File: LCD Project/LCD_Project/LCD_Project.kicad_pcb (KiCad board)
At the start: 2 copper layers, 109 x 88.5 mm, 6 parts, among them J1 DT15-4P, U1 Teensy4.0, U2 MIC5365-1.3YC5-TR

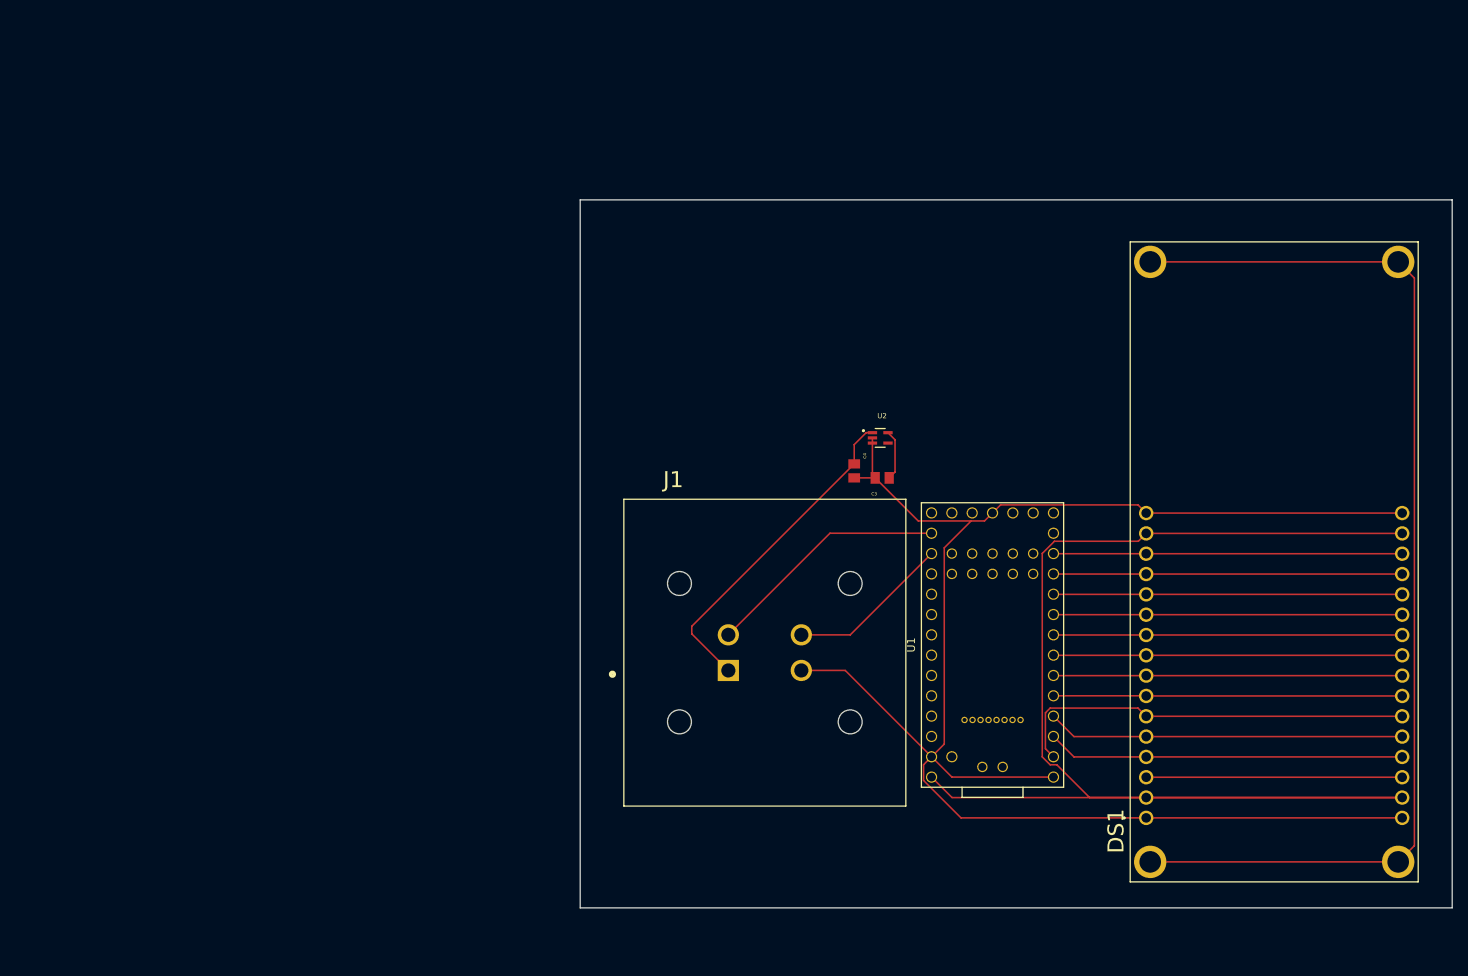
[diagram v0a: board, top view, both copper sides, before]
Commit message: Add files via upload
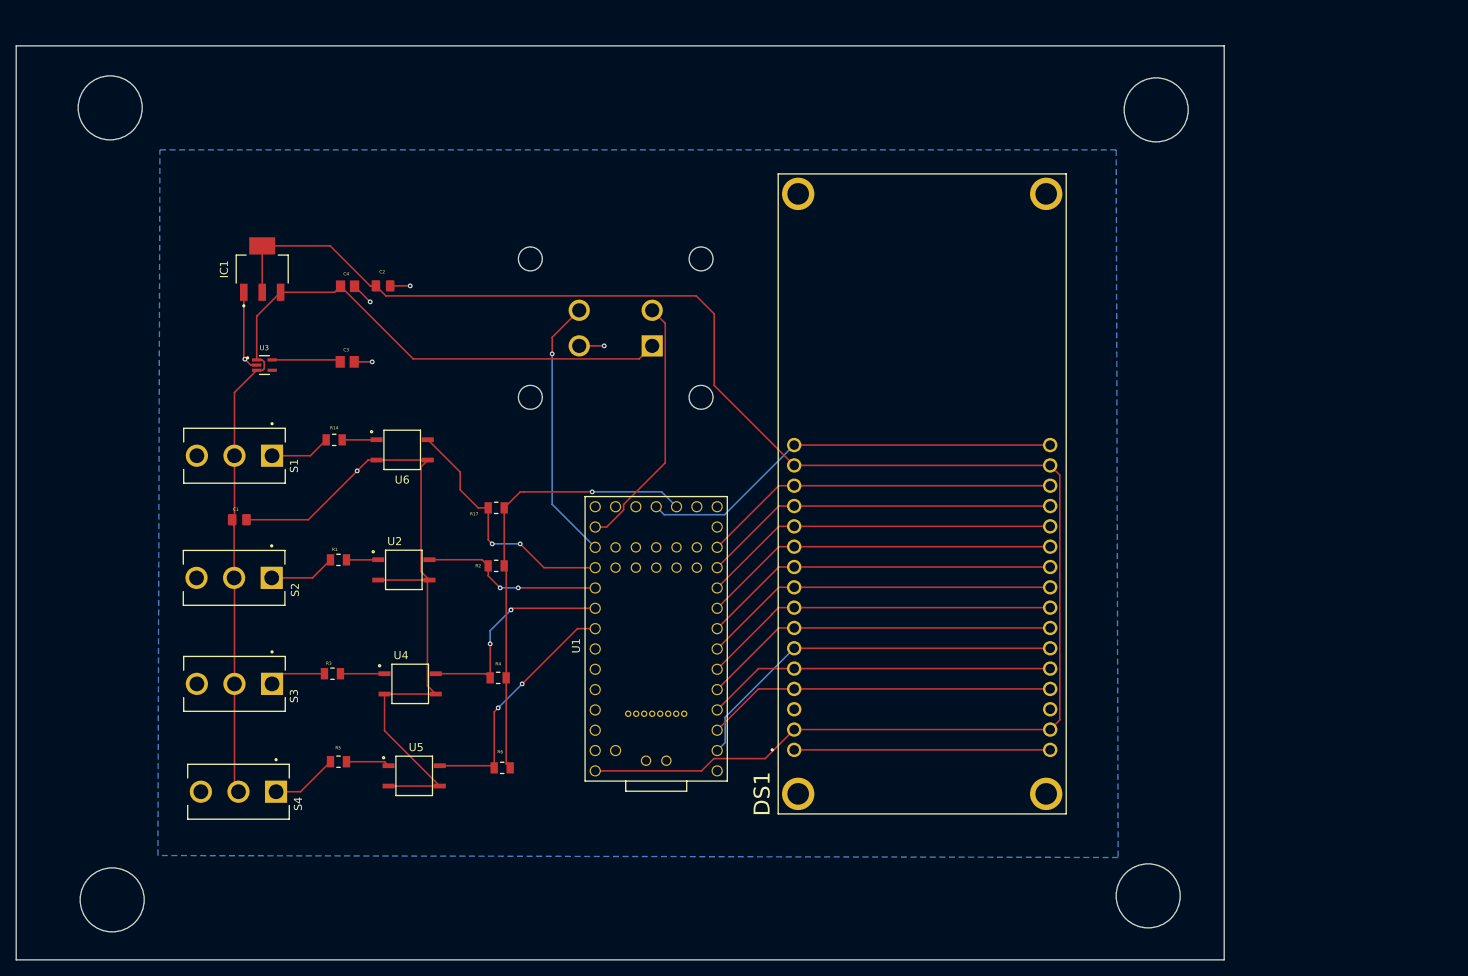
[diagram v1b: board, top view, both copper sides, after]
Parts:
- added C1: CL21A106KOQNNNE, CL21A106KOQNNNE:CAPC2012X140N, F.Cu at (102.4, 84.5)
- added C2: CL21A106KOQNNNE, CL21A106KOQNNNE:CAPC2012X140N, F.Cu at (120.4, 55.2)
- added IC1: REG1117-5, REG1117-5:SOT230P700X180-4N, F.Cu at (105.2, 53.1)
- added R1: 10K, CRCW08051K00FKEA:RESC2012X50N, F.Cu at (114.8, 89.5)
- added R14: 10K, CRCW08051K00FKEA:RESC2012X50N, F.Cu at (114.2, 74.5)
- added R17: 10K, CRCW08051K00FKEA:RESC2012X50N, F.Cu at (134.5, 83.0)
- added R2: 10K, CRCW08051K00FKEA:RESC2012X50N, F.Cu at (134.5, 90.2)
- added R3: 10K, CRCW08051K00FKEA:RESC2012X50N, F.Cu at (114.0, 103.7)
- added R4: 10K, CRCW08051K00FKEA:RESC2012X50N, F.Cu at (134.8, 104.2)
- added R5: 10K, CRCW08051K00FKEA:RESC2012X50N, F.Cu at (114.8, 114.7)
- added R6: 10K, CRCW08051K00FKEA:RESC2012X50N, F.Cu at (135.2, 115.5)
- added S1: 100SP1T1B4M2QE, 100SP1T1B4M2QE:SW_100SP1T1B4M2QE, F.Cu at (101.8, 76.5)
- added S2: 100SP1T1B4M2QE, 100SP1T1B4M2QE:SW_100SP1T1B4M2QE, F.Cu at (101.7, 91.8)
- added S3: 100SP1T1B4M2QE, 100SP1T1B4M2QE:SW_100SP1T1B4M2QE, F.Cu at (101.8, 105.0)
- added S4: 100SP1T1B4M2QE, 100SP1T1B4M2QE:SW_100SP1T1B4M2QE, F.Cu at (102.3, 118.5)
- added U3: MIC5365-1.3YC5-TR, MIC5365-1.3YC5-TR:SOT65P210X110-5N, F.Cu at (105.5, 65.2)
- added U4: VOM618A-3T, VOM618A-3T:SOIC254P695X242-4N, F.Cu at (123.8, 105.0)
- added U5: VOM618A-3T, VOM618A-3T:SOIC254P695X242-4N, F.Cu at (124.2, 116.5)
- added U6: VOM618A-3T, VOM618A-3T:SOIC254P695X242-4N, F.Cu at (122.8, 75.8)
- J1: moved to B.Cu
- U2: value MIC5365-1.3YC5-TR -> VOM618A-3T; footprint MIC5365-1.3YC5-TR:SOT65P210X110-5N -> VOM618A-3T:SOIC254P695X242-4N
- moved C3 68.4 mm to (115.9, 64.8), turned to 0 degrees
- moved C4 67.4 mm to (115.9, 55.3), turned to 0 degrees
- moved U2 61.8 mm to (123.0, 90.8)
- moved DS1 44.8 mm to (187.8, 81.2)
- moved J1 44.6 mm to (149.4, 60.5), turned to 180 degrees
- moved U1 42.0 mm to (154.5, 99.4)
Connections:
- DS1 pad 3_1: Net-(DS1-V0-Pad3_1) -> unconnected-(DS1-V0-Pad3_1)_1
- DS1 pad 3_2: Net-(DS1-V0-Pad3_1) -> unconnected-(DS1-V0-Pad3_1)
- DS1 pad S1: Net-(DS1-SHIELD-PadS1) -> unconnected-(DS1-SHIELD-PadS1)_3
- DS1 pad S2: Net-(DS1-SHIELD-PadS1) -> unconnected-(DS1-SHIELD-PadS1)_1
- DS1 pad S3: Net-(DS1-SHIELD-PadS1) -> unconnected-(DS1-SHIELD-PadS1)_2
- DS1 pad S4: Net-(DS1-SHIELD-PadS1) -> unconnected-(DS1-SHIELD-PadS1)
- U1 pad 16: unconnected-(U1-3V3-Pad16) -> +3.3V
- U1 pad 23: unconnected-(U1-16_A2_RX4_SCL1-Pad23) -> Net-(U1-16_A2_RX4_SCL1)
- U1 pad 24: unconnected-(U1-17_A3_TX4_SDA1-Pad24) -> Net-(U1-17_A3_TX4_SDA1)
- U1 pad 25: unconnected-(U1-18_A4_SDA0-Pad25) -> Net-(U1-18_A4_SDA0)
- U1 pad 26: unconnected-(U1-19_A5_SCL0-Pad26) -> Net-(U1-19_A5_SCL0)
- U2 pad 1: +12V -> Net-(R1-Pad2)
- U2 pad 4: (no net) -> Net-(U1-17_A3_TX4_SDA1)
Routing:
- net Net-(DS1-SHIELD-PadS1): track 138.7 -> 0.00 mm
- net +12V: track 41.4 -> 118.1 mm
- net +3.3V: track 0.00 -> 55.9 mm, vias 0 -> 1
- net +5V: track 178.5 -> 213.9 mm
- net Net-(DS1-V0-Pad3_1): track 32.0 -> 0.00 mm
- net Net-(U1-16_A2_RX4_SCL1): track 0.00 -> 31.2 mm, vias 0 -> 2
- net Net-(U1-19_A5_SCL0): track 0.00 -> 30.8 mm, vias 0 -> 2
- net Net-(U1-18_A4_SDA0): track 0.00 -> 27.2 mm, vias 0 -> 2
- net Net-(U1-17_A3_TX4_SDA1): track 0.00 -> 22.9 mm, vias 0 -> 2
- net GND: track 210.8 -> 196.0 mm, vias 0 -> 6
- net Net-(U1-15_A1_RX3_SPDIF_IN): track 20.5 -> 33.3 mm, vias 0 -> 1
- net Net-(R5-Pad1): track 0.00 -> 8.35 mm
- net Net-(R1-Pad1): track 0.00 -> 8.28 mm
- net Net-(R14-Pad1): track 0.00 -> 7.59 mm
- net Net-(R3-Pad1): track 0.00 -> 7.08 mm
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- added copper zone on B.Cu, net GND
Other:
- board size 109 x 88.5 mm -> 151 x 114.2 mm

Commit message: Add files via upload
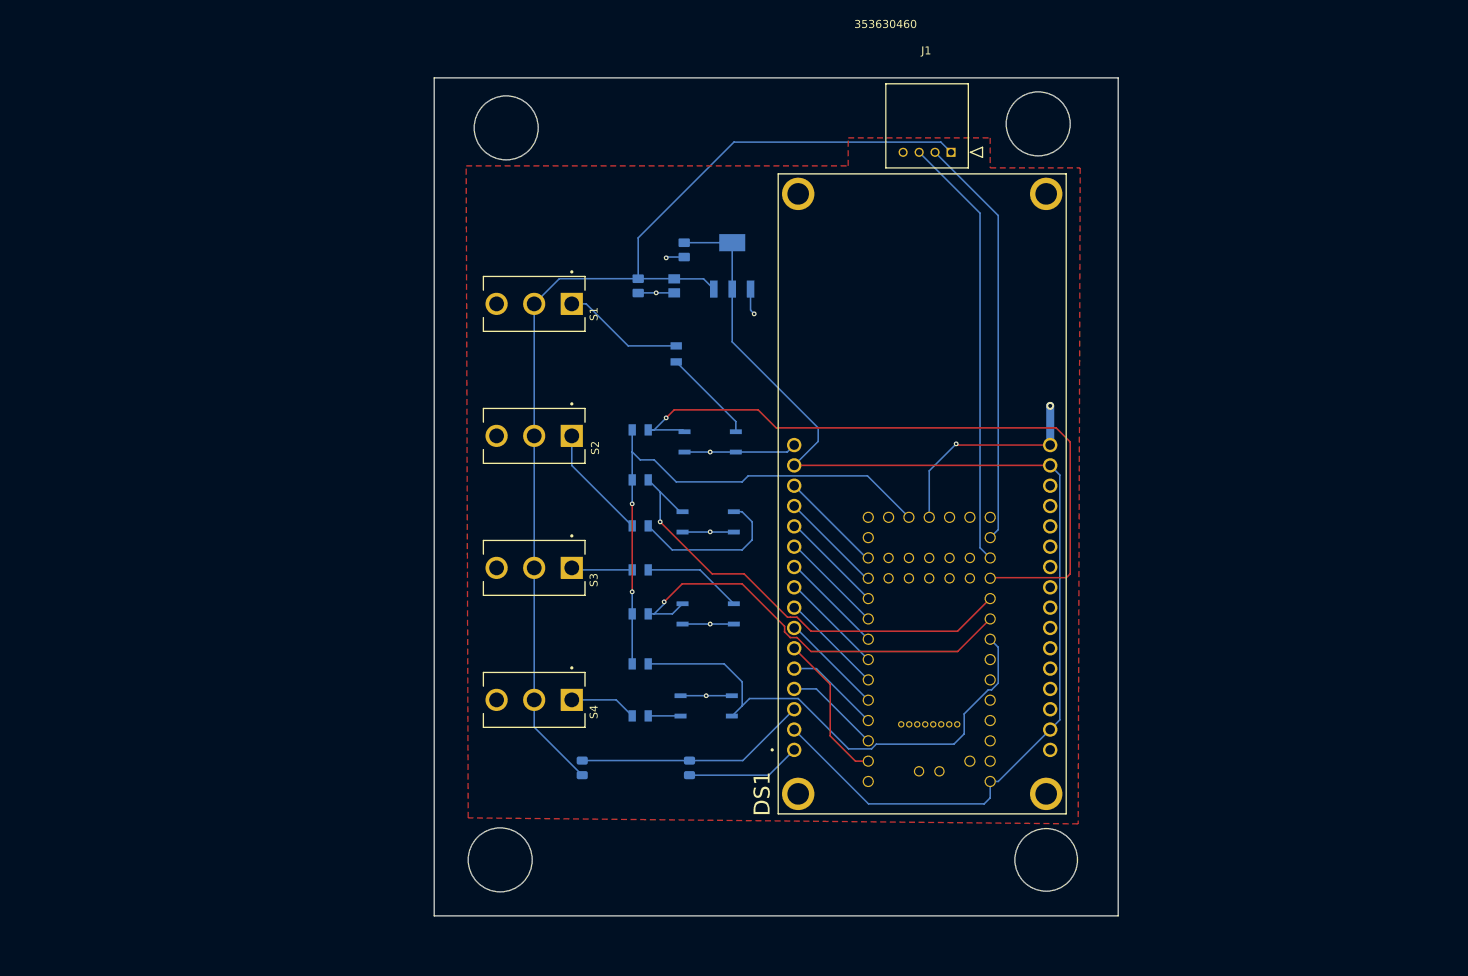
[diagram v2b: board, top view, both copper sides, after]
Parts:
- removed C3: C0805C104Z3VACTU, C0805C104Z3VACTU:CAPC2012X88N
- removed U3: MIC5365-1.3YC5-TR, MIC5365-1.3YC5-TR:SOT65P210X110-5N
- added R7: R_250, Resistor_SMD:R_0805_2012Metric, B.Cu at (145.2, 115.5)
- added R8: R_110, Resistor_SMD:R_0805_2012Metric, B.Cu at (158.7, 115.5)
- C1, C2, C4, IC1, R1, R14, R17, R2, R3, R4, R5, R6, U1, U2, U4, U5, U6: moved to B.Cu
- J1: value DT15-4P -> 353630460; footprint DT15-4P:TE_DT15-4P -> 353630460:CON_353630460; moved to F.Cu
- moved IC1 58.8 mm to (164.0, 52.8)
- moved C1 57.8 mm to (152.2, 55.2), turned to -90 degrees
- moved J1 47.3 mm to (191.4, 38.6), turned to 0 degrees
- moved R14 44.1 mm to (157.0, 63.8), turned to -90 degrees
- moved S1 42.0 mm to (139.2, 57.5)
- moved S2 41.5 mm to (139.2, 74.0)
- moved C4 40.8 mm to (156.8, 55.2), turned to -90 degrees
- moved R3 40.6 mm to (152.5, 90.8)
- moved S3 40.2 mm to (139.2, 90.5)
- moved S4 38.7 mm to (139.2, 107.0)
- moved U2 38.5 mm to (161.0, 84.8), turned to 180 degrees
- moved U6 38.5 mm to (161.2, 74.8), turned to 180 degrees
- moved U4 38.3 mm to (161.0, 96.2), turned to 180 degrees
- moved R5 38.1 mm to (152.5, 109.0)
- moved R1 38.0 mm to (152.5, 85.2)
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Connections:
- DS1 pad 3_1: unconnected-(DS1-V0-Pad3_1)_1 -> +3.7V
- DS1 pad 3_2: unconnected-(DS1-V0-Pad3_1) -> +3.7V
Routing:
- net GND: track 196.0 -> 85.2 mm, vias 6 -> 9
- net +5V: track 213.9 -> 146.4 mm
- net Net-(U1-16_A2_RX4_SCL1): track 31.2 -> 86.8 mm, vias 2 -> 1
- net Net-(U1-17_A3_TX4_SDA1): track 22.9 -> 58.3 mm, vias 2 -> 1
- net Net-(U1-19_A5_SCL0): track 30.8 -> 63.3 mm, vias 2 -> 0
- net Net-(U1-7_RX2_OUT1A): track 44.9 -> 13.0 mm
- net Net-(U1-9_OUT1C): track 44.9 -> 13.0 mm
- net Net-(U1-5_IN2): track 44.8 -> 13.0 mm
- net Net-(U1-4_BCLK2): track 44.8 -> 13.0 mm
- net Net-(U1-8_TX2_IN1): track 44.8 -> 13.0 mm
- net Net-(U1-6_OUT1D): track 44.8 -> 13.0 mm
- net Net-(U1-3_LRCLK2): track 44.8 -> 13.0 mm
- net Net-(U1-2_OUT2): track 43.8 -> 11.9 mm
- net Net-(U1-1_TX1_CTX2_MISO1): track 43.8 -> 11.9 mm
- net Net-(U1-10_CS_MQSR): track 44.8 -> 13.0 mm
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- added copper zone on F.Cu, net GND
- removed copper zone on B.Cu, net GND
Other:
- board size 151 x 114.2 mm -> 85.5 x 104.8 mm
